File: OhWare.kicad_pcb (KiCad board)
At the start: 2 copper layers, 100 x 105.4 mm, 49 parts, among them J1 Screw_Terminal_01x03, J10 Conn_02x15_Odd_Even, J11 Conn_01x04_Pin, J2 Conn_01x03_Pin, J3 Conn_01x02_Pin, J4 Conn_01x03_Pin, J7 Conn_01x06_Pin, J8 Conn_01x04_Pin, J9 Conn_02x10_Odd_Even, SW1 SW_DIP_x01, SW2 SW_DIP_x01, SW3 SW_DIP_x01, U10 SP3485EN-L/TR, U2 SIT65HVD230DR, U3 SIT3490EESA, U4 XL1509-5.0E1, U5 AMS1117-3.3, U6 AMS1117-3.3, U7 ESP32-WROOM-32

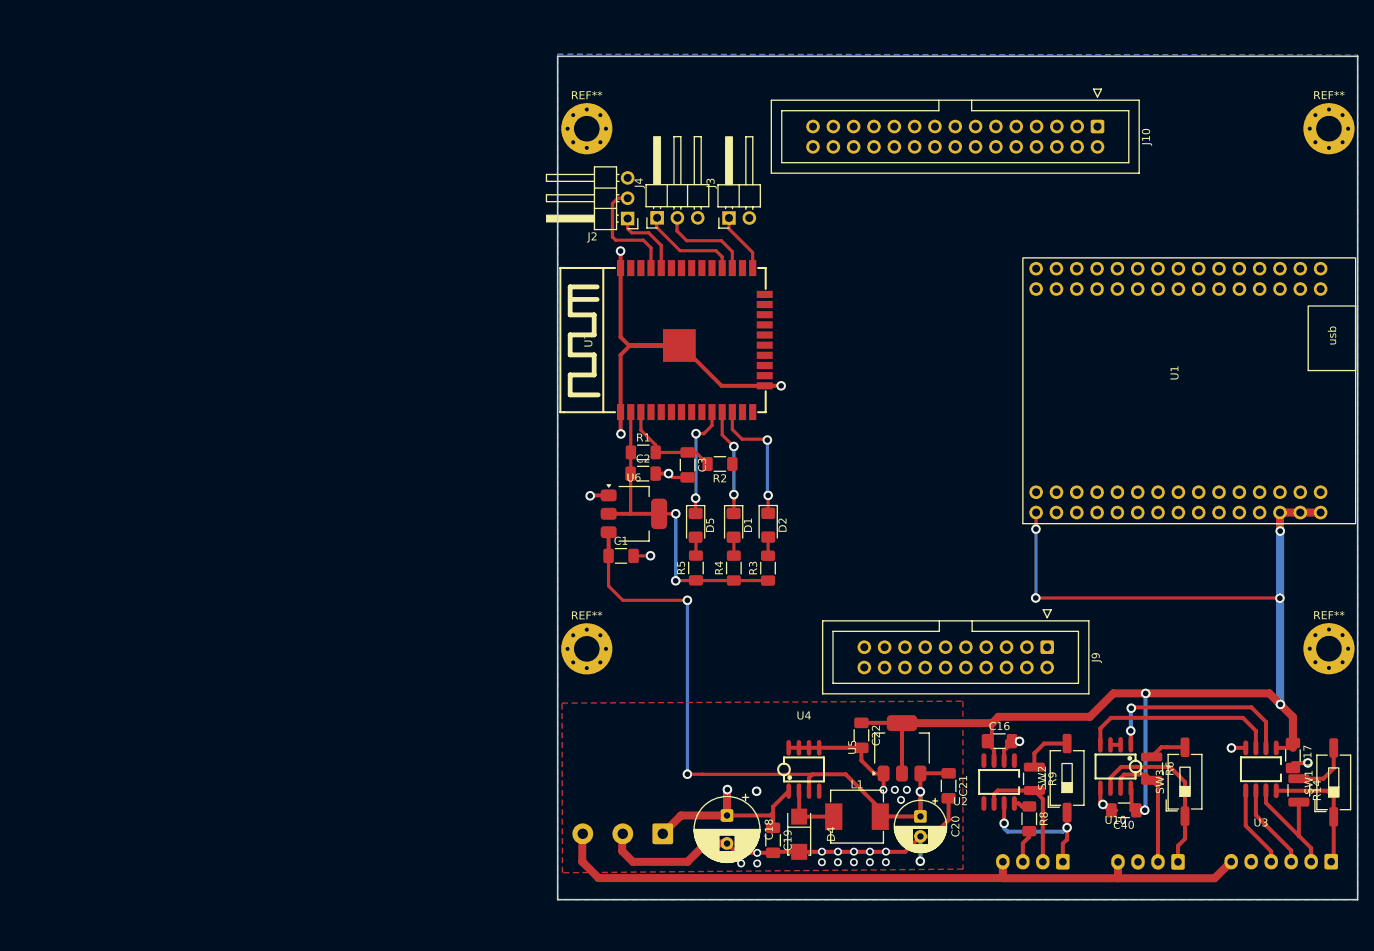
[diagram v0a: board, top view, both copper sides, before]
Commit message: Latest Changes
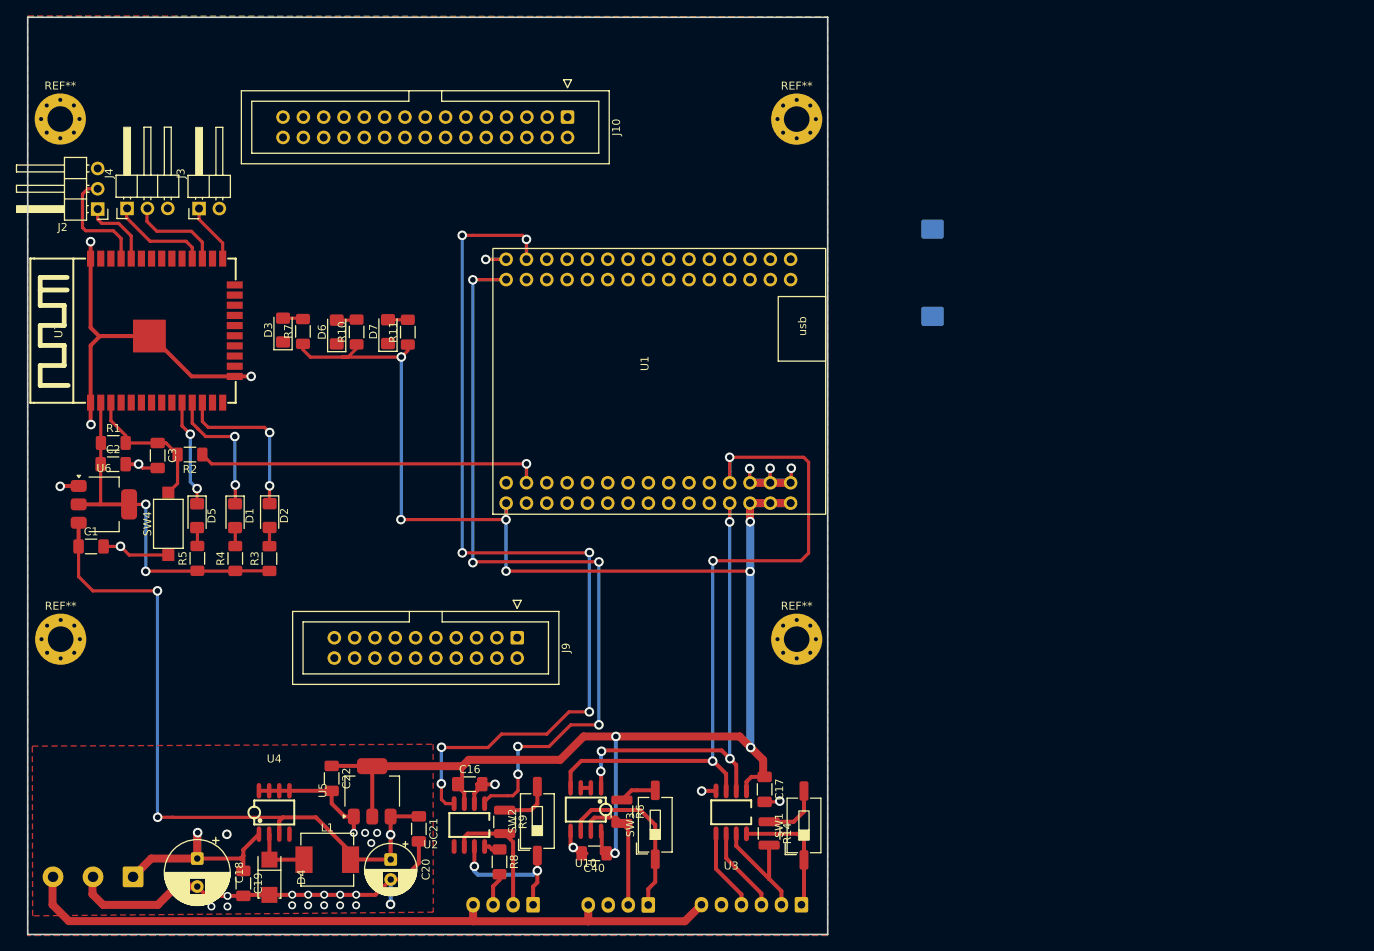
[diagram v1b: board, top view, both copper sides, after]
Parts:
- added D3: LED, LED_SMD:LED_1206_3216Metric_Pad1.42x1.75mm_HandSolder, F.Cu at (65.7, 78.8)
- added D6: LED, LED_SMD:LED_1206_3216Metric_Pad1.42x1.75mm_HandSolder, F.Cu at (72.4, 79.0)
- added D7: LED, LED_SMD:LED_1206_3216Metric_Pad1.42x1.75mm_HandSolder, F.Cu at (78.8, 79.0)
- added JP1: Jumper_2_Bridged, Jumper:Jumper_Harwin_S1621_P10.9mm, B.Cu at (146.9, 71.6)
- added R10: 1k, Resistor_SMD:R_1206_3216Metric_Pad1.30x1.75mm_HandSolder, F.Cu at (74.9, 79.0)
- added R11: 1k, Resistor_SMD:R_1206_3216Metric_Pad1.30x1.75mm_HandSolder, F.Cu at (81.3, 79.1)
- added R7: 1k, Resistor_SMD:R_1206_3216Metric_Pad1.30x1.75mm_HandSolder, F.Cu at (68.2, 79.0)
- added SW4: SW_Push, Button_Switch_SMD:SW_SPST_CK_RS282G05A3, F.Cu at (51.3, 103.0)
- moved REF** 66.5 mm to (129.9, 52.4)
- moved REF** 66.5 mm to (129.9, 117.4)
- moved C18 66.4 mm to (55.0, 144.9)
- moved J8 66.4 mm to (96.9, 150.6)
- moved R14 66.4 mm to (126.4, 141.7)
- moved R6 66.4 mm to (108.0, 139.0)
- moved SW2 66.4 mm to (97.5, 140.2)
- moved U10 66.4 mm to (103.5, 138.7)
- moved U2 66.4 mm to (89.0, 140.7)
- moved C16 66.4 mm to (89.0, 135.6)
- moved C19 66.4 mm to (60.7, 148.0)
- moved C20 66.4 mm to (79.1, 145.0)
- moved C21 66.4 mm to (82.7, 141.2)
- moved C22 66.4 mm to (71.8, 134.8)
- moved C40 66.4 mm to (104.6, 144.2)
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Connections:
- net /Esp32/SPI_CLK renamed /Controller/SPI3_SCK
- net /Esp32/SPI_MOSI renamed /Controller/SPI3_MOSI
- R2 pad 1: /Esp32/EN -> /Controller/SPI3_DEN
- U1 pad 23: unconnected-(U1-B11-Pad23) -> /Controller/USART3_RX
- U1 pad 24: unconnected-(U1-B10-Pad24) -> /Controller/USART3_TX
- U1 pad 31: unconnected-(U1-B9-Pad31) -> /CAN/CAN_TXD
- U1 pad 34: unconnected-(U1-B8-Pad34) -> /CAN/CAN_RXD
- U1 pad 4: unconnected-(U1-C13-Pad4) -> /Controller/SPI3_DEN
- U10 pad 1: /RS485/RO -> /Controller/USART3_RX
- U10 pad 4: /RS485/DI -> /Controller/USART3_TX
- U3 pad 2: /RS485/RO -> /Controller/USART3_RX
- U3 pad 3: /RS485/DI -> /Controller/USART3_TX
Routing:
- net /CAN/CAN_RXD: track 0.00 -> 117.4 mm, vias 0 -> 7
- net /CAN/CAN_TXD: track 0.00 -> 102.0 mm, vias 0 -> 6
- net /Controller/USART3_TX: track 0.00 -> 90.1 mm, vias 0 -> 3
- net +3.3V: track 163.4 -> 228.6 mm, vias 7 -> 9
- net /Controller/USART3_RX: track 0.00 -> 59.8 mm, vias 0 -> 4
- net /Controller/SPI3_DEN: track 0.00 -> 45.7 mm, vias 0 -> 1
- net GND: track 144.4 -> 177.7 mm, vias 30 -> 34
- net /RS485/RO: track 25.5 -> 0.00 mm, vias 2 -> 0
- net /RS485/DI: track 24.8 -> 0.00 mm
- net +5V: track 85.3 -> 91.8 mm
- net Net-(U7-EN): track 12.9 -> 18.1 mm
- net +3.3VESP: track 41.1 -> 45.4 mm
- net /Esp32/INDESP_LED2: track 16.3 -> 20.3 mm
- net /Esp32/INDESP_LED1: track 13.3 -> 17.0 mm
- net Net-(D3-A): track 0.00 -> 2.53 mm
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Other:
- board size 100 x 105.4 mm -> 100 x 114.7 mm
